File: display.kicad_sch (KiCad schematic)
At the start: 1 part, among them J3 AXF5D3012

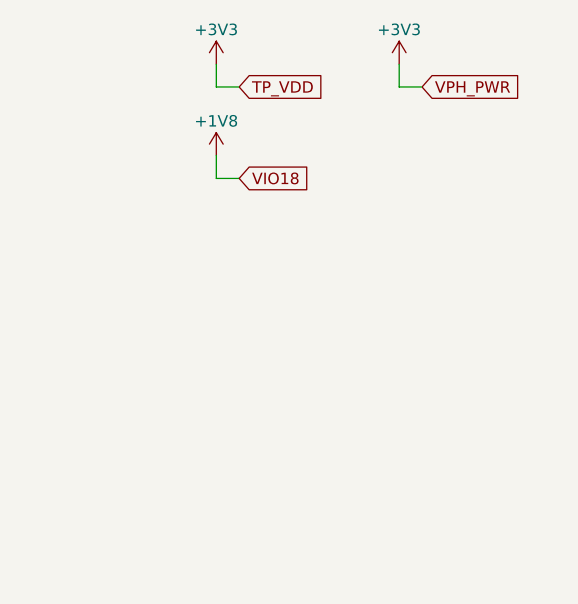
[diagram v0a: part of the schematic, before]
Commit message: added buck
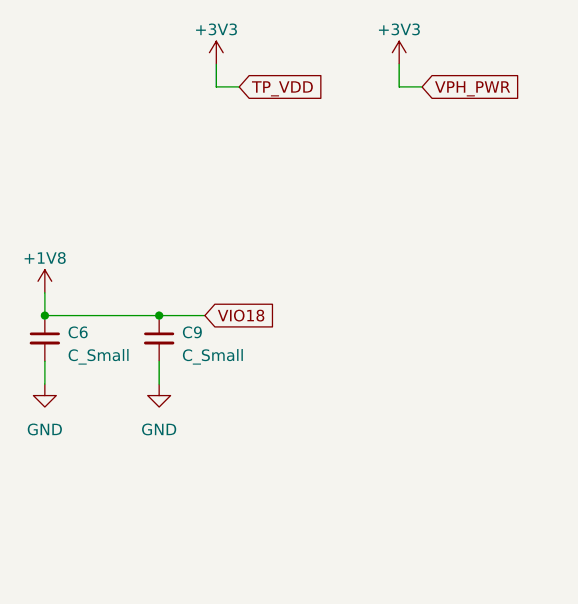
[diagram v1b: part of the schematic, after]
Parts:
- added C6, C9: C_Small, symbol Device:C_Small
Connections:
- net +1V8: now also C6.1, C9.1
- net GND: now also C6.2, C9.2
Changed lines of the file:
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@@
 (kicad_sch (version 20230121) (generator eeschema)
   (paper "A4")
+  (junction (at 33.02 69.85) (diameter 0) (color 0 0 0 0)
+  )
   (junction (at 139.7 127) (diameter 0) (color 0 0 0 0)
   )
   (junction (at 137.16 63.5) (diameter 0) (color 0 0 0 0)
   )
+  (junction (at 45.72 69.85) (diameter 0) (color 0 0 0 0)
+  )
   (junction (at 143.51 63.5) (diameter 0) (color 0 0 0 0)
   )
@@
     (stroke (width 0) (type default))
   )
-  (wire (pts (xy 52.07 52.07) (xy 52.07 54.61))
-    (stroke (width 0) (type default))
-  )
   (wire (pts (xy 168.91 95.25) (xy 171.45 95.25))
     (stroke (width 0) (type default))
@@
     (stroke (width 0) (type default))
   )
+  (wire (pts (xy 33.02 67.31) (xy 33.02 69.85))
+    (stroke (width 0) (type default))
+  )
   (wire (pts (xy 137.16 63.5) (xy 139.7 63.5))
     (stroke (width 0) (type default))
@@
     (stroke (width 0) (type default))
   )
-  (wire (pts (xy 54.61 54.61) (xy 52.07 54.61))
-    (stroke (width 0) (type default))
-  )
   (wire (pts (xy 137.16 63.5) (xy 137.16 66.04))
     (stroke (width 0) (type default))
@@
     (stroke (width 0) (type default))
   )
+  (wire (pts (xy 45.72 69.85) (xy 50.8 69.85))
+    (stroke (width 0) (type default))
+  )
   (wire (pts (xy 110.49 90.17) (xy 113.03 90.17))
     (stroke (width 0) (type default))
@@
     (stroke (width 0) (type default))
   )
+  (wire (pts (xy 33.02 69.85) (xy 45.72 69.85))
+    (stroke (width 0) (type default))
+  )
   (wire (pts (xy 110.49 97.79) (xy 113.03 97.79))
     (stroke (width 0) (type default))
   )
+  (wire (pts (xy 33.02 74.93) (xy 33.02 77.47))
+    (stroke (width 0) (type default))
+  )
   (wire (pts (xy 139.7 124.46) (xy 139.7 127))
     (stroke (width 0) (type default))
@@
   )
   (wire (pts (xy 52.07 41.91) (xy 52.07 44.45))
+    (stroke (width 0) (type default))
+  )
+  (wire (pts (xy 45.72 74.93) (xy 45.72 77.47))
     (stroke (width 0) (type default))
   )
@@
     )
   )
-  (global_label "VIO18" (shape input) (at 54.61 54.61 0) (fields_autoplaced)
-    (effects (font (size 1.27 1.27)) (justify left))
-    (property "Intersheetrefs" "${INTERSHEET_REFS}" (at 62.9587 54.61 0)
-      (effects (font (size 1.27 1.27)) (justify left) hide)
-    )
-  )
   (global_label "NFC_ANT2" (shape input) (at 110.49 105.41 180) (fields_autoplaced)
     (effects (font (size 1.27 1.27)) (justify right))
@@
     )
   )
+  (global_label "VIO18" (shape input) (at 50.8 69.85 0) (fields_autoplaced)
+    (effects (font (size 1.27 1.27)) (justify left))
+    (property "Intersheetrefs" "${INTERSHEET_REFS}" (at 59.1487 69.85 0)
+      (effects (font (size 1.27 1.27)) (justify left) hide)
+    )
+  )
   (global_label "VPH_PWR" (shape input) (at 137.16 60.96 90) (fields_autoplaced)
     (effects (font (size 1.27 1.27)) (justify left))
@@
     )
   )
+  (symbol (lib_id "power:+1V8") (at 33.02 67.31 0) (unit 1)
+    (in_bom yes) (on_board yes) (dnp no) (fields_autoplaced)
+    (property "Reference" "#PWR028" (at 33.02 71.12 0)
+      (effects (font (size 1.27 1.27)) hide)
+    )
+    (property "Value" "+1V8" (at 33.02 63.5 0)
+      (effects (font (size 1.27 1.27)))
+    )
+    (property "Footprint" "" (at 33.02 67.31 0)
+      (effects (font (size 1.27 1.27)) hide)
+    )
+    (property "Datasheet" "" (at 33.02 67.31 0)
+      (effects (font (size 1.27 1.27)) hide)
+    )
+    (pin "1")
+    (instances
+      (project "armband"
+        (path "/017c50c6-333c-4d31-ad5a-278994a09b14"
+          (reference "#PWR028") (unit 1)
+        )
+        (path "/017c50c6-333c-4d31-ad5a-278994a09b14/ae5dc462-dca9-40e4-ba02-6b87a86a4904"
+          (reference "#PWR028") (unit 1)
+        )
+        (path "/017c50c6-333c-4d31-ad5a-278994a09b14/ea4ffdec-697e-4619-8bda-0f4c7cf70f55"
+          (reference "#PWR028") (unit 1)
+        )
+      )
+    )
+  )
   (symbol (lib_id "power:+3V3") (at 52.07 41.91 0) (unit 1)
     (in_bom yes) (on_board yes) (dnp no) (fields_autoplaced)
@@
         )
         (path "/017c50c6-333c-4d31-ad5a-278994a09b14/ea4ffdec-697e-4619-8bda-0f4c7cf70f55"
-          (reference "#PWR010") (unit 1)
+          (reference "#PWR013") (unit 1)
+        )
+      )
+    )
+  )
+  (symbol (lib_id "Device:C_Small") (at 45.72 72.39 0) (mirror y) (unit 1)
+    (in_bom yes) (on_board yes) (dnp no) (fields_autoplaced)
+    (property "Reference" "C9" (at 48.26 71.7613 0)
+      (effects (font (size 1.27 1.27)) (justify right))
+    )
+    (property "Value" "C_Small" (at 48.26 74.3013 0)
+      (effects (font (size 1.27 1.27)) (justify right))
+    )
+    (property "Footprint" "" (at 45.72 72.39 0)
+      (effects (font (size 1.27 1.27)) hide)
+    )
+    (property "Datasheet" "~" (at 45.72 72.39 0)
+      (effects (font (size 1.27 1.27)) hide)
+    )
+    (pin "1")
+    (pin "2")
+    (instances
+      (project "armband"
+        (path "/017c50c6-333c-4d31-ad5a-278994a09b14"
+          (reference "C9") (unit 1)
+        )
+        (path "/017c50c6-333c-4d31-ad5a-278994a09b14/ae5dc462-dca9-40e4-ba02-6b87a86a4904"
+          (reference "C9") (unit 1)
+        )
+        (path "/017c50c6-333c-4d31-ad5a-278994a09b14/ea4ffdec-697e-4619-8bda-0f4c7cf70f55"
+          (reference "C9") (unit 1)
         )
       )
@@
         )
         (path "/017c50c6-333c-4d31-ad5a-278994a09b14/ea4ffdec-697e-4619-8bda-0f4c7cf70f55"
-          (reference "#PWR012") (unit 1)
-        )
-      )
-    )
-  )
-  (symbol (lib_id "power:+1V8") (at 52.07 52.07 0) (unit 1)
-    (in_bom yes) (on_board yes) (dnp no) (fields_autoplaced)
-    (property "Reference" "#PWR087" (at 52.07 55.88 0)
-      (effects (font (size 1.27 1.27)) hide)
-    )
-    (property "Value" "+1V8" (at 52.07 48.26 0)
-      (effects (font (size 1.27 1.27)))
-    )
-    (property "Footprint" "" (at 52.07 52.07 0)
-      (effects (font (size 1.27 1.27)) hide)
-    )
-    (property "Datasheet" "" (at 52.07 52.07 0)
-      (effects (font (size 1.27 1.27)) hide)
-    )
-    (pin "1")
-    (instances
-      (project "armband"
-        (path "/017c50c6-333c-4d31-ad5a-278994a09b14"
-          (reference "#PWR087") (unit 1)
-        )
-        (path "/017c50c6-333c-4d31-ad5a-278994a09b14/ea4ffdec-697e-4619-8bda-0f4c7cf70f55"
-          (reference "#PWR011") (unit 1)
+          (reference "#PWR015") (unit 1)
+        )
+      )
+    )
+  )
+  (symbol (lib_id "power:GND") (at 33.02 77.47 0) (unit 1)
+    (in_bom yes) (on_board yes) (dnp no) (fields_autoplaced)
+    (property "Reference" "#PWR029" (at 33.02 83.82 0)
+      (effects (font (size 1.27 1.27)) hide)
+    )
+    (property "Value" "GND" (at 33.02 82.55 0)
+      (effects (font (size 1.27 1.27)))
+    )
+    (property "Footprint" "" (at 33.02 77.47 0)
+      (effects (font (size 1.27 1.27)) hide)
+    )
+    (property "Datasheet" "" (at 33.02 77.47 0)
+      (effects (font (size 1.27 1.27)) hide)
+    )
+    (pin "1")
+    (instances
+      (project "armband"
+        (path "/017c50c6-333c-4d31-ad5a-278994a09b14"
+          (reference "#PWR029") (unit 1)
+        )
+        (path "/017c50c6-333c-4d31-ad5a-278994a09b14/ae5dc462-dca9-40e4-ba02-6b87a86a4904"
+          (reference "#PWR029") (unit 1)
+        )
+        (path "/017c50c6-333c-4d31-ad5a-278994a09b14/ea4ffdec-697e-4619-8bda-0f4c7cf70f55"
+          (reference "#PWR029") (unit 1)
         )
       )
@@
         )
         (path "/017c50c6-333c-4d31-ad5a-278994a09b14/ea4ffdec-697e-4619-8bda-0f4c7cf70f55"
-          (reference "#PWR013") (unit 1)
+          (reference "#PWR016") (unit 1)
         )
       )
@@
         )
       )
+    )
+  )
+  (symbol (lib_id "power:GND") (at 45.72 77.47 0) (unit 1)
+    (in_bom yes) (on_board yes) (dnp no) (fields_autoplaced)
+    (property "Reference" "#PWR032" (at 45.72 83.82 0)
+      (effects (font (size 1.27 1.27)) hide)
+    )
+    (property "Value" "GND" (at 45.72 82.55 0)
+      (effects (font (size 1.27 1.27)))
+    )
+    (property "Footprint" "" (at 45.72 77.47 0)
+      (effects (font (size 1.27 1.27)) hide)
+    )
+    (property "Datasheet" "" (at 45.72 77.47 0)
+      (effects (font (size 1.27 1.27)) hide)
+    )
+    (pin "1")
+    (instances
+      (project "armband"
+        (path "/017c50c6-333c-4d31-ad5a-278994a09b14"
+          (reference "#PWR032") (unit 1)
+        )
+        (path "/017c50c6-333c-4d31-ad5a-278994a09b14/ae5dc462-dca9-40e4-ba02-6b87a86a4904"
+          (reference "#PWR032") (unit 1)
+        )
+        (path "/017c50c6-333c-4d31-ad5a-278994a09b14/ea4ffdec-697e-4619-8bda-0f4c7cf70f55"
+          (reference "#PWR032") (unit 1)
+        )
+      )
+    )
+  )
+  (symbol (lib_id "Device:C_Small") (at 33.02 72.39 0) (mirror y) (unit 1)
+    (in_bom yes) (on_board yes) (dnp no) (fields_autoplaced)
+    (property "Reference" "C6" (at 35.56 71.7613 0)
+      (effects (font (size 1.27 1.27)) (justify right))
+    )
+    (property "Value" "C_Small" (at 35.56 74.3013 0)
+      (effects (font (size 1.27 1.27)) (justify right))
+    )
+    (property "Footprint" "" (at 33.02 72.39 0)
+      (effects (font (size 1.27 1.27)) hide)
+    )
+    (property "Datasheet" "~" (at 33.02 72.39 0)
+      (effects (font (size 1.27 1.27)) hide)
+    )
+    (pin "1")
+    (pin "2")
+    (instances
+      (project "armband"
+        (path "/017c50c6-333c-4d31-ad5a-278994a09b14"
+          (reference "C6") (unit 1)
+        )
+        (path "/017c50c6-333c-4d31-ad5a-278994a09b14/ae5dc462-dca9-40e4-ba02-6b87a86a4904"
+          (reference "C6") (unit 1)
+        )
+        (path "/017c50c6-333c-4d31-ad5a-278994a09b14/ea4ffdec-697e-4619-8bda-0f4c7cf70f55"
+          (reference "C6") (unit 1)
+        )
+      )
